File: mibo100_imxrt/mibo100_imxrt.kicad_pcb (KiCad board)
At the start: 2 copper layers, 53 parts, among them J1 Conn_01x26, J2 Conn_01x26, J3 Conn_02x02_Odd_Even, J4 USB_B_Micro, J5 Conn_01x05, SW1 SW_Push, U1 MIMXRT1021CAF4A, U2 W25X80, U3 AP3417C, Y1 24MHz

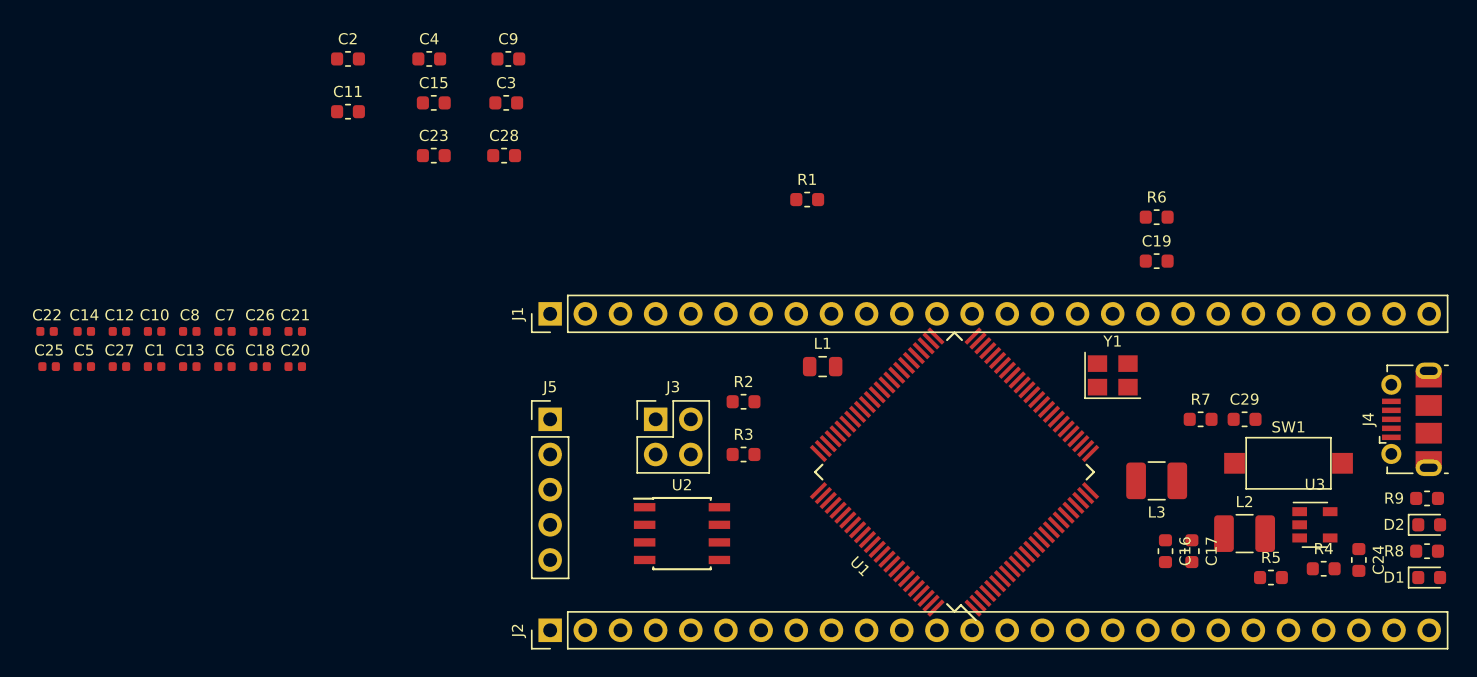
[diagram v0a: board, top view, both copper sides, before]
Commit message: routing finished
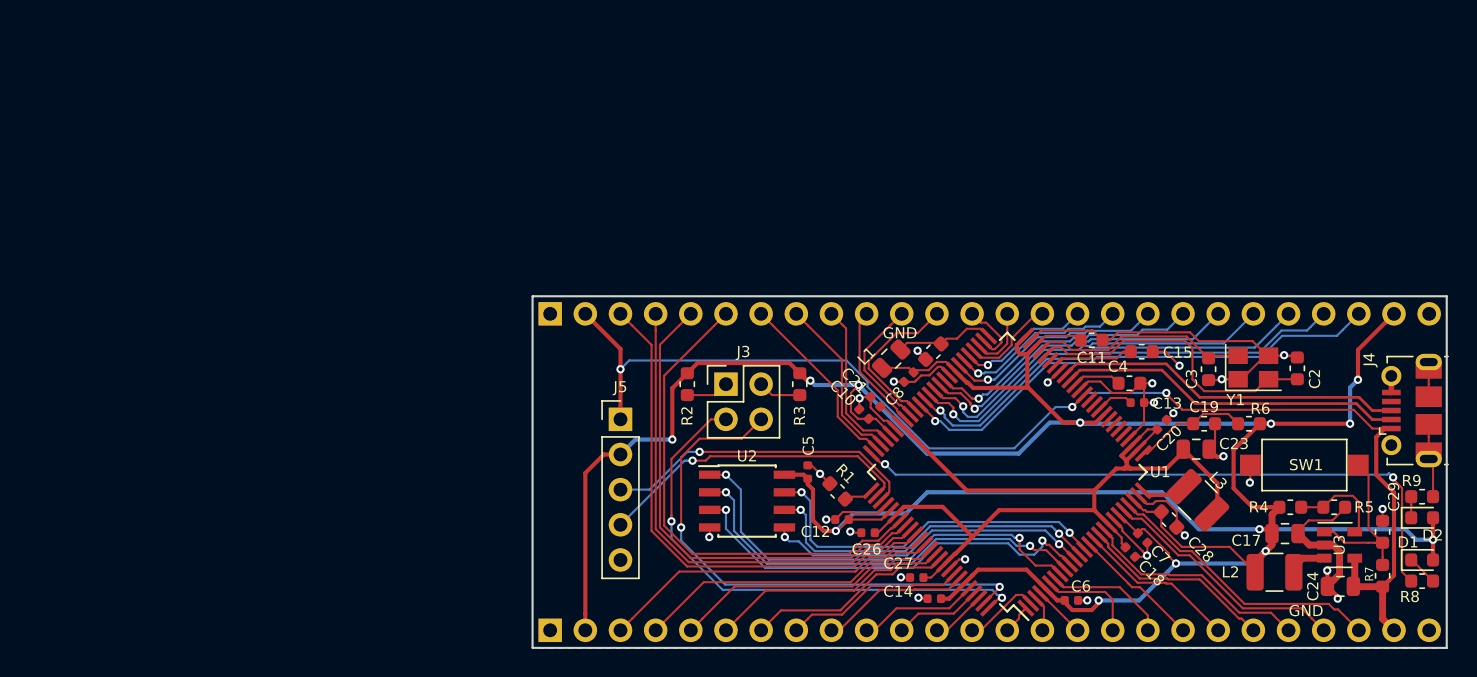
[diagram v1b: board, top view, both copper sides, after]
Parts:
- removed C1, C22, C25: 220nF, Capacitor_SMD:C_0402_1005Metric
- removed C16: 100nF, Capacitor_SMD:C_0603_1608Metric
- C17, C23, C24: footprint Capacitor_SMD:C_0603_1608Metric -> Capacitor_SMD:C_0805_2012Metric
- J1, J2: moved to B.Cu
- L2, L3: footprint Inductor_SMD:L_1210_3225Metric_Pad1.42x2.65mm_HandSolder -> Inductor_SMD:L_1210_3225Metric
- moved C2 72.1 mm to (165.7, 75.1), turned to 90 degrees
- moved C13 68.5 mm to (154.2, 77.5)
- moved C7 68.0 mm to (154.6, 87.3), turned to 315 degrees
- moved C14 64.4 mm to (139.5, 91.7), turned to 180 degrees
- moved C18 64.3 mm to (153.7, 88.3), turned to 315 degrees
- moved C6 63.4 mm to (149.4, 91.8)
- moved C20 62.8 mm to (156.0, 79.1), turned to 45 degrees
- moved C27 59.6 mm to (138.2, 90.2), turned to 180 degrees
- moved C23 59.0 mm to (158.4, 80.9)
- moved C11 56.2 mm to (150.9, 73.0)
- moved C4 55.7 mm to (153.6, 76.1)
- moved C28 54.8 mm to (156.5, 86.0), turned to 315 degrees
- moved C3 54.3 mm to (159.3, 75.1), turned to 270 degrees
- moved C15 54.2 mm to (154.5, 73.9)
- moved C12 53.9 mm to (132.8, 86.0), turned to 180 degrees
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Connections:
- J1 pad 10: /E25 -> /E20
- J1 pad 11: /E26 -> /E19
- J1 pad 12: /E27 -> /E18
- J1 pad 13: /E32 -> /E8
- J1 pad 14: /E33 -> /E9
- J1 pad 15: /E34 -> /E7
- J1 pad 16: /E35 -> /E6
- J1 pad 17: /B10 -> /E5
- J1 pad 18: /B11 -> /E4
- J1 pad 19: /B12 -> /S5
- J1 pad 20: /B13 -> /S4
- J1 pad 21: /B14 -> /S3
- J1 pad 22: /B15 -> /S2
- J1 pad 23: /E4 -> /S1
- J1 pad 24: /E5 -> /S0
- J1 pad 3: /E18 -> /E27
- J1 pad 4: /E19 -> /E26
- J1 pad 5: /E20 -> /E25
- J1 pad 6: /E21 -> /E24
- J1 pad 7: /E22 -> /E23
- J1 pad 8: /E23 -> /E22
- J1 pad 9: /E24 -> /E21
- J2 pad 10: /A11 -> /A7
- J2 pad 11: /A12 -> /A8
- J2 pad 12: /A13 -> /A9
- J2 pad 13: /A14 -> /B15
- J2 pad 14: /A15 -> /B14
- J2 pad 15: /S0 -> /B13
- J2 pad 16: /S1 -> /B12
- J2 pad 17: /S2 -> /B11
- J2 pad 18: /S3 -> /B10
- J2 pad 19: /S4 -> /A15
- J2 pad 20: /S5 -> /A14
- J2 pad 21: /E6 -> /A13
- J2 pad 22: /E7 -> /A12
- J2 pad 23: /E8 -> /A11
- J2 pad 24: /E9 -> /A10
- J2 pad 3: /A4 -> /E32
- J2 pad 4: /A5 -> /E33
- J2 pad 5: /A6 -> /E34
- J2 pad 6: /A7 -> /E35
- J2 pad 7: /A8 -> /A4
- J2 pad 8: /A9 -> /A5
- J2 pad 9: /A10 -> /A6
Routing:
- net +3V3: track 0.00 -> 240.9 mm, vias 0 -> 13
- net GND: track 0.00 -> 102.3 mm, vias 0 -> 25
- net /5V: track 0.00 -> 92.9 mm, vias 0 -> 3
- net /DCDC_OUT: track 0.00 -> 67.9 mm
- net /LED1: track 0.00 -> 46.5 mm, vias 0 -> 2
- net /BOOT-CFG-1: track 0.00 -> 39.0 mm, vias 0 -> 2
- net /BOOT-CFG-0: track 0.00 -> 37.8 mm, vias 0 -> 2
- net /E32: track 0.00 -> 37.7 mm
- net /E35: track 0.00 -> 36.1 mm
- net /E34: track 0.00 -> 36.0 mm
- net /A10: track 0.00 -> 36.0 mm, vias 0 -> 1
- net /E33: track 0.00 -> 35.9 mm
- net /A11: track 0.00 -> 33.0 mm, vias 0 -> 1
- net /FLASH-CS: track 0.00 -> 32.0 mm, vias 0 -> 2
- net /FLASH-D2: track 0.00 -> 31.0 mm, vias 0 -> 2
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- added copper zone on B.Cu, net GND
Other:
- board outline added: 66 x 25.4 mm
- net class Default: clearance 0.2 -> 0.152; trace_width 0.25 -> 0.152; via_dia 0.8 -> 0.6; via_drill 0.4 -> 0.3
- net class USB_HS added: clearance 0.152, trace_width 0.21, via_dia 0.6, via_drill 0.3
- rule trace_clearance: 0.2 -> 0.152
- rule trace_min: 0.2 -> 0.152
- board text added: "GND"
